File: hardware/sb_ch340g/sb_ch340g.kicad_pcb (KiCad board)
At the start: 2 copper layers, 45.7 x 35.6 mm, 14 parts, among them P1 USB_OTG, P2 CONN_01X06, P3 CONN_01X13, P4 CONN_01X13, U1 AMS1117-3.3, U2 CH340G, U3 RF200, Y1 12MHz

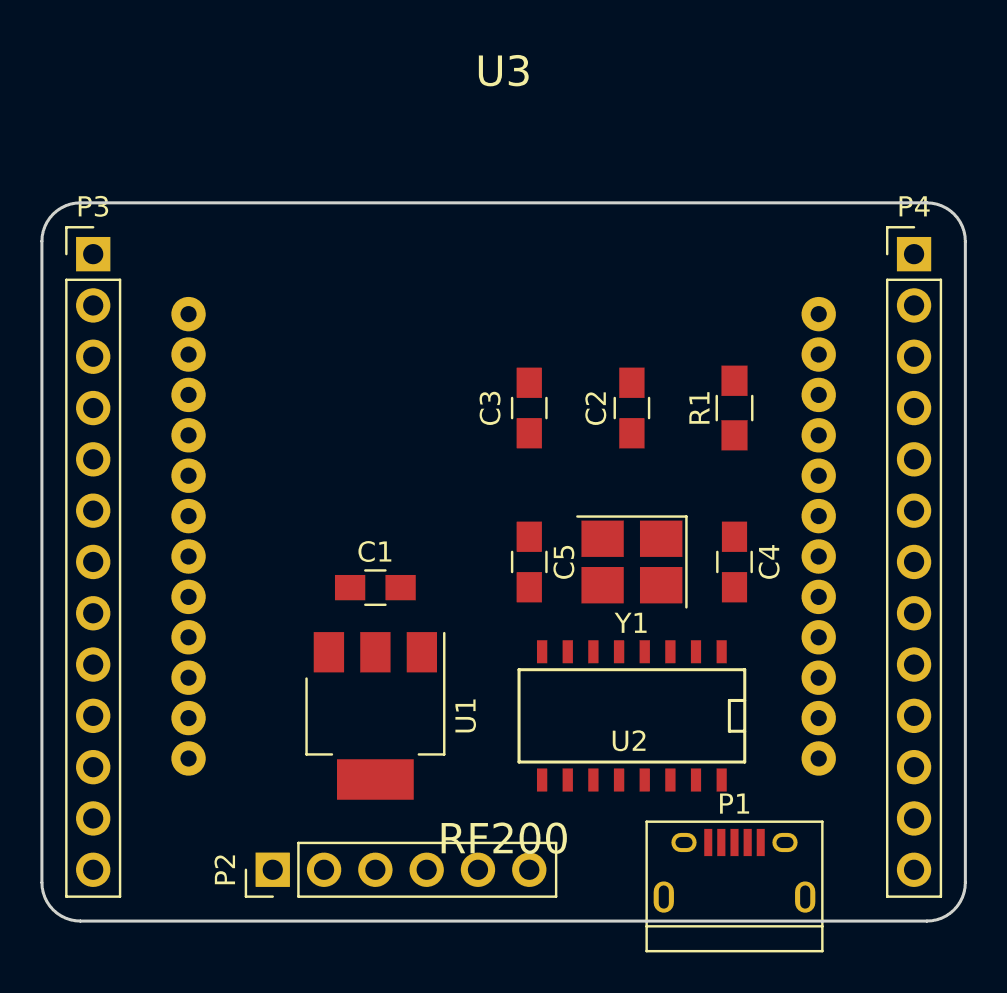
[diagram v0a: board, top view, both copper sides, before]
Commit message: Cleanup layout.
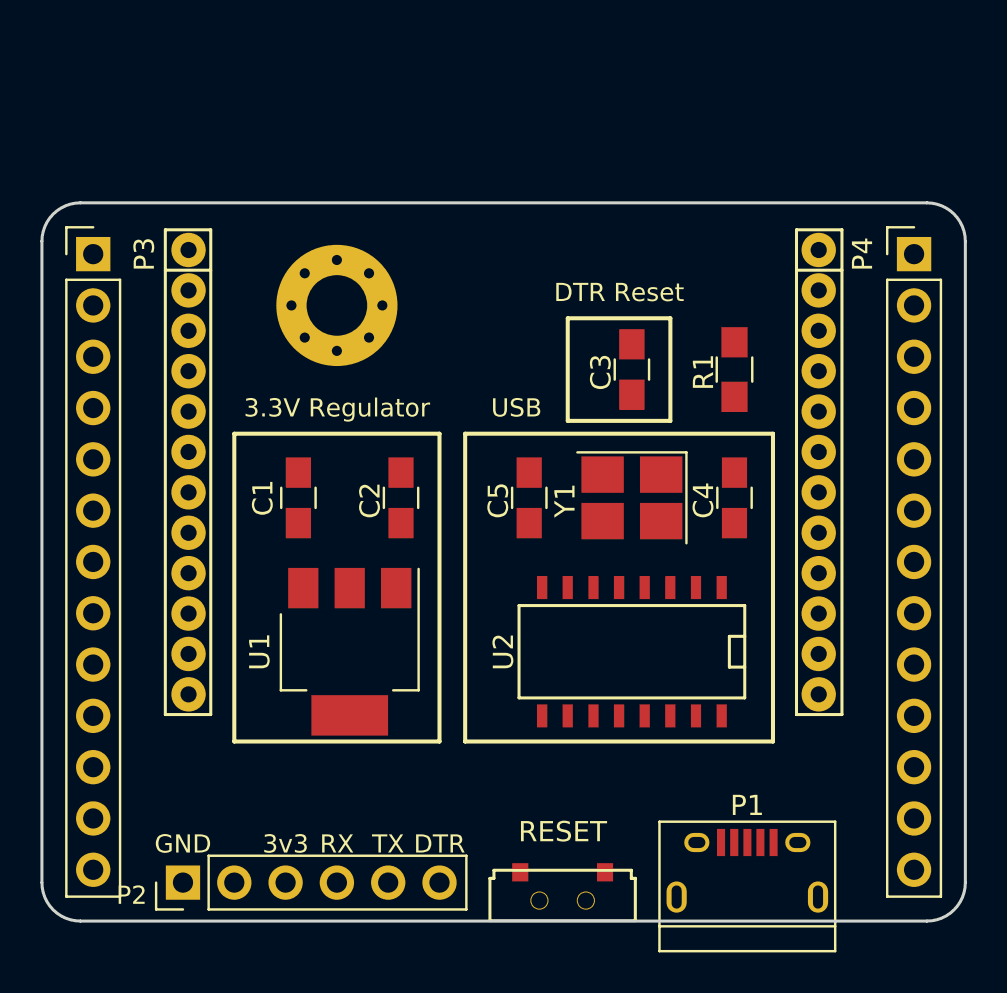
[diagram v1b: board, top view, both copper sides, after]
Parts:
- added REF**: MountingHole_3mm_Pad_Via, Mounting_Holes:MountingHole_3mm_Pad_Via, F.Cu at (140.3, 91.4)
- added RESET: RESET_SW, CrumpPrints:3x6x3.5mm_side_pushbutton_smd, F.Cu at (151.5, 120.9)
- U3: footprint CrumpPrints:RF200_nosilk -> CrumpPrints:RF200
- moved C2 12.3 mm to (143.5, 101.0)
- moved C1 5.85 mm to (138.4, 101.0), turned to 90 degrees
- moved C3 5.43 mm to (154.9, 94.6)
- moved P2 4.49 mm to (132.7, 120.0)
- moved U1 3.42 mm to (141.0, 108.6)
- moved U2 3.18 mm to (154.9, 108.6)
- moved U3 3.18 mm to (148.6, 99.7)
- moved C4 3.17 mm to (160.0, 101.0)
- moved C5 3.17 mm to (149.9, 101.0)
- moved Y1 3.17 mm to (154.9, 101.0)
- moved R1 1.91 mm to (160.0, 94.6)
- moved P1 0.63 mm to (160.7, 119.4)
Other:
- board text added: "3.3V Regulator"
- board text added: "3v3"
- board text added: "DTR"
- board text added: "DTR Reset"
- board text added: "GND"
- board text added: "RX"
- board text added: "TX"
- board text added: "USB"
